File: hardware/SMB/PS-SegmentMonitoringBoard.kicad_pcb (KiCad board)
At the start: 4 copper layers, 83.9 x 80.3 mm, 121 parts, among them IC1 BQ79616PAPR, J1 voltTapsConn, J2 highSideConn, J3 lowSideConn, J4 thermsConn, Q1 ZXTN4004KTC

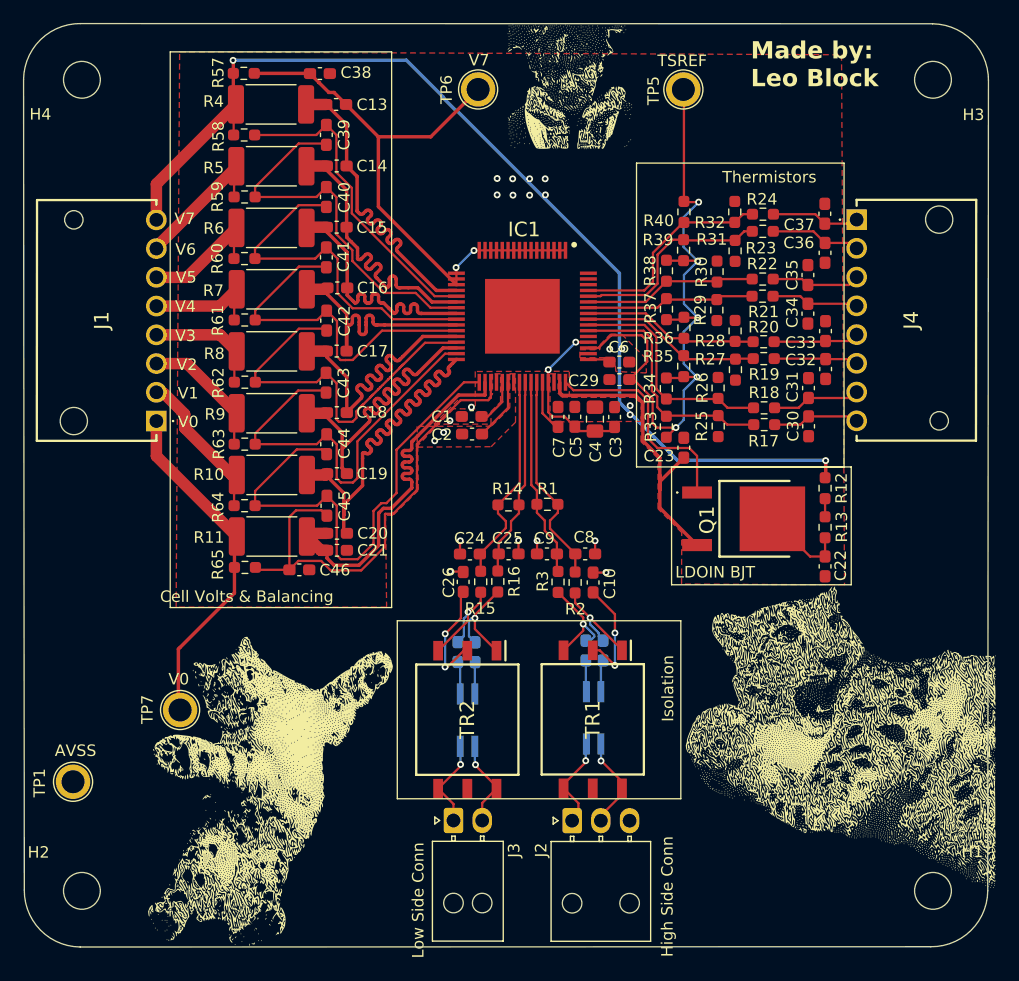
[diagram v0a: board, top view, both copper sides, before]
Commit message: more ss updates
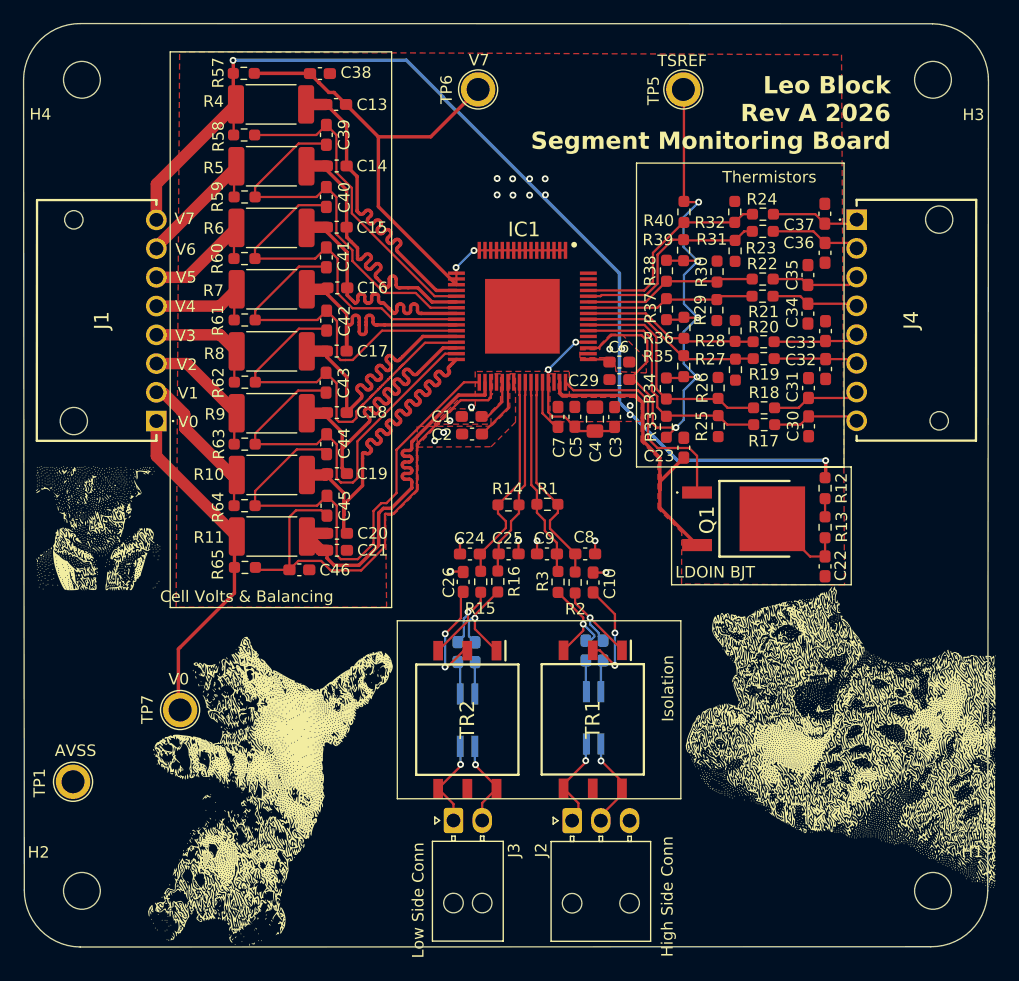
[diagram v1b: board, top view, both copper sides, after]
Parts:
- moved G*** 56.2 mm to (80.6, 106.9)
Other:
- board text added: "Leo Block Rev A 2026 Segment Monitoring Board"
- board text removed: "Made by: Leo Block"
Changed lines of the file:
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@@
 	(footprint "LOGO"
 		(layer "F.Cu")
-		(at 121.630192 68.538834)
+		(at 80.600192 106.928834)
 		(property "Reference" "G***"
 			(at 0 0 0)
@@
 		)
 	)
-	(gr_text "Made by:\nLeo Block\n"
-		(at 137.36 68.67 0)
+	(gr_text "Leo Block\nRev A 2026\nSegment Monitoring Board"
+		(at 149.54 74.12 0)
 		(layer "F.SilkS")
 		(effects
@@
 				(bold yes)
 			)
-			(justify left bottom)
+			(justify right bottom)
 		)
 	)
